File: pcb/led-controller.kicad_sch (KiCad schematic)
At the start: 39 parts, among them J1 BOOT_SEL, J2 Programmer Conn, J3 USB_C_Receptacle, SW1 PD Reset, U1 STM32F411CCUx, U2 STUSB4500QTR, Y1 16MHz

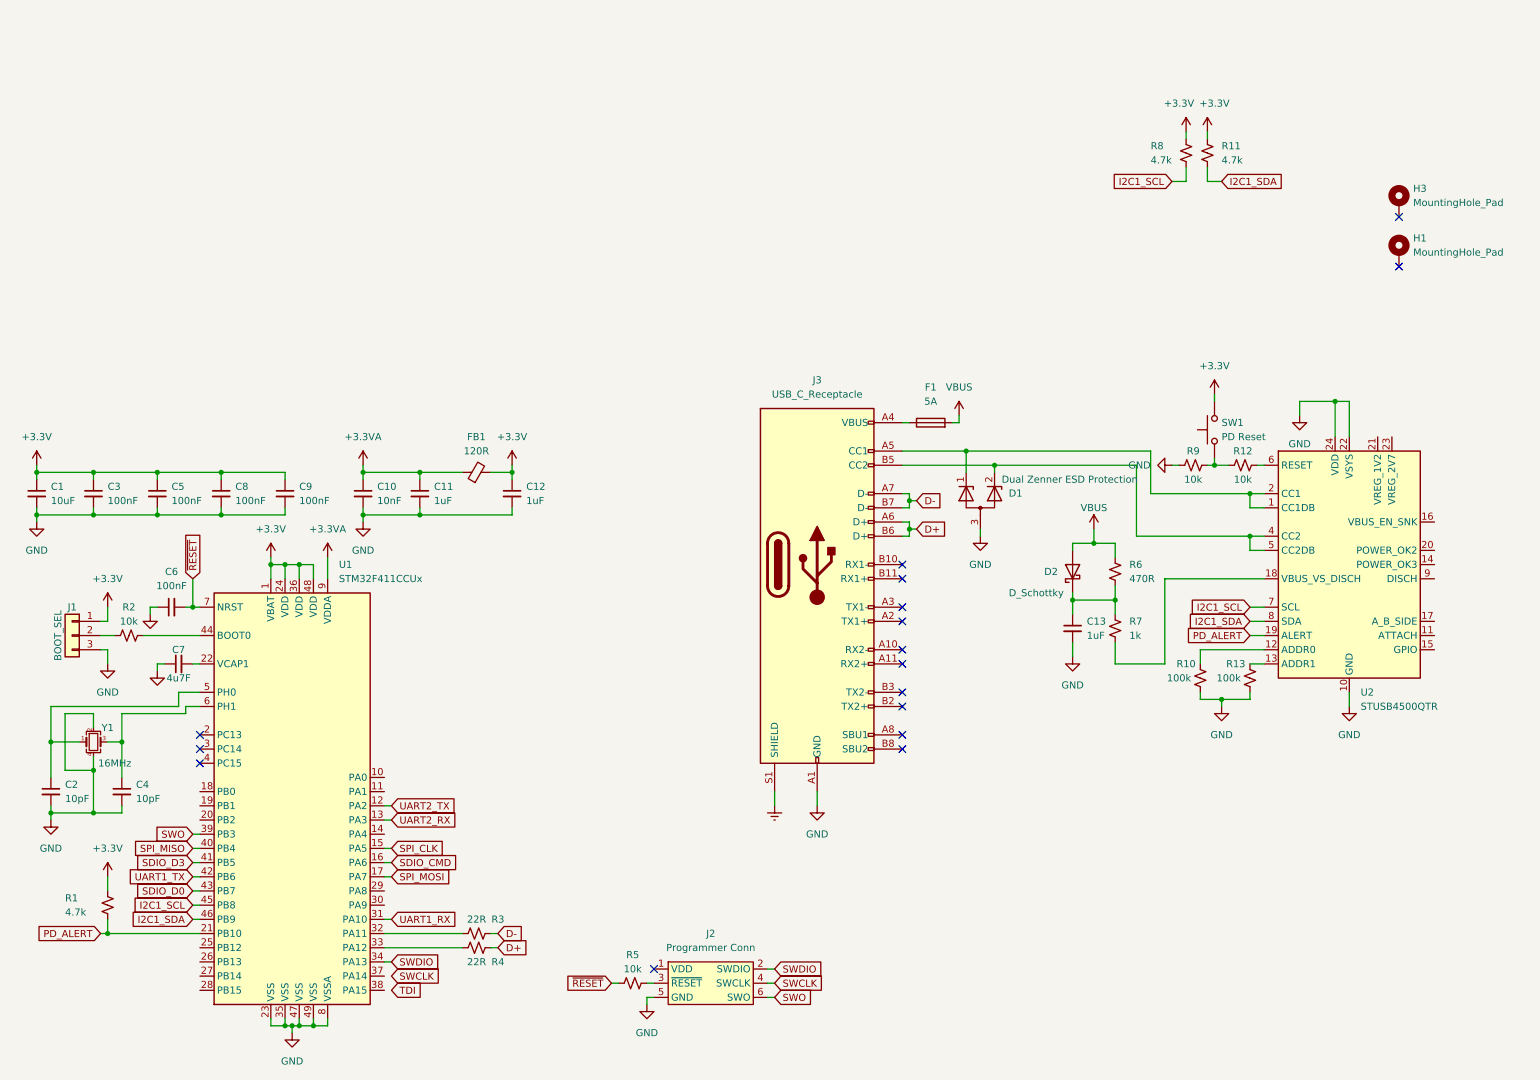
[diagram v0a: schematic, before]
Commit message: PCB updates
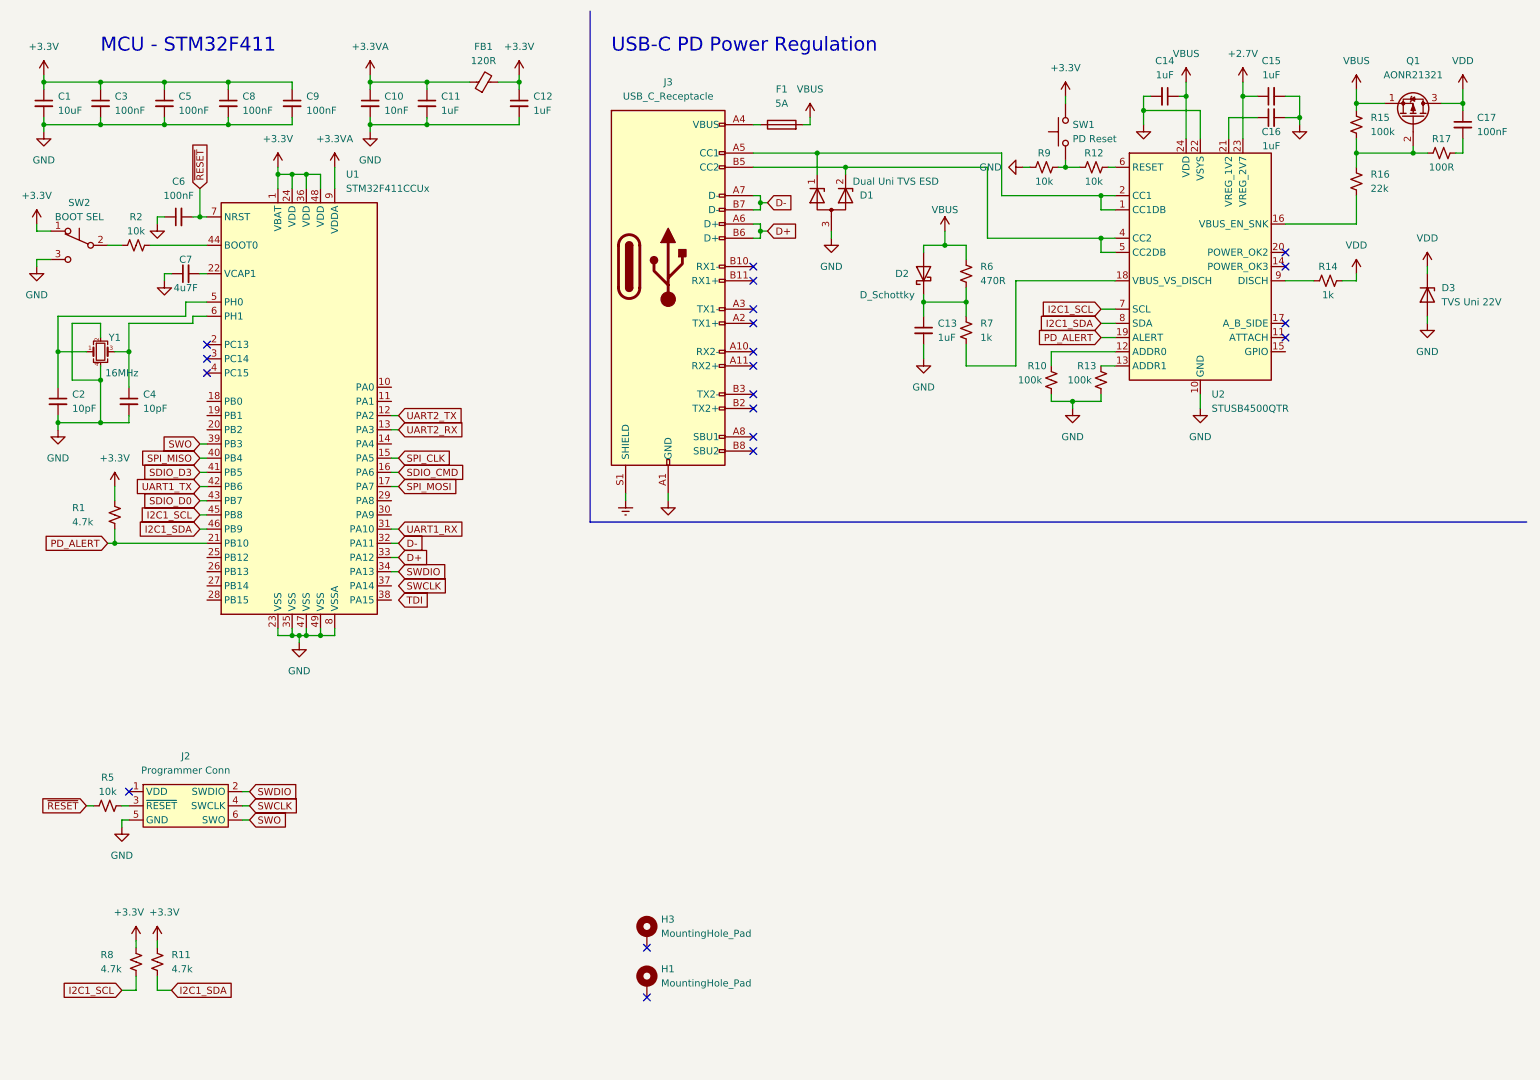
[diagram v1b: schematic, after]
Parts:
- removed J1: BOOT_SEL, Connector_PinHeader_1.27mm:PinHeader_1x03_P1.27mm_Horizontal, symbol Connector_Generic:Conn_01x03
- removed R3, R4: 22R, Resistor_SMD:R_0603_1608Metric, symbol Device:R_Small_US
- added C14, C15, C16: 1uF, Capacitor_SMD:C_0603_1608Metric, symbol Device:C_Small
- added C17: 100nF, Capacitor_SMD:C_0603_1608Metric, symbol Device:C_Small
- added D3: TVS Uni 22V, symbol Device:D_Zener
- added Q1: AONR21321, ATL:AONR21321, symbol ATL:AONR21321
- added R14: 1k, Resistor_SMD:R_0603_1608Metric, symbol Device:R_Small_US
- added R15: 100k, Resistor_SMD:R_0603_1608Metric, symbol Device:R_Small_US
- added R16: 22k, Resistor_SMD:R_0603_1608Metric, symbol Device:R_Small_US
- added R17: 100R, Resistor_SMD:R_0603_1608Metric, symbol Device:R_Small_US
- added SW2: BOOT SEL, Button_Switch_SMD:SW_DIP_SPSTx01_Slide_Copal_CVS-01xB_W5.9mm_P1mm, symbol Switch:SW_Push_SPDT
- D1: value Dual Zenner ESD Protection -> Dual Uni TVS ESD
- F1: footprint (none) -> ATL:Littlefuse-154
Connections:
- net +3.3V: now also SW2.1 (A)
- net D+: now also U1.33 (PA12)
- net D-: now also U1.32 (PA11)
- net GND: now also C14.2, C15.2, C16.2, D3.2 (A), SW2.3 (C); no longer U2.24 (VDD)
- net VBUS: now also U2.24 (VDD), C14.1, Q1.1 (S), R15.1
- net at R2.1: now also SW2.2 (B)
- net at U2.16 (VBUS_EN_SNK): now also R16.2
- net at U2.21 (VREG_1V2): now also C16.1
- net +2V7: now reaches U2.23 (VREG_2V7)
- net +2V7: now also C15.1
- net at U2.9 (DISCH): now also R14.1
- new net: Q1.2 (G), R15.2, R16.1, R17.1
- new net: C17.2, R17.2
- new net VDD: C17.1, D3.1 (K), Q1.3 (D), R14.2
- no-connect marks 16 -> 20
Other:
- note added: "MCU - STM32F411"
- note added: "USB-C PD Power Regulation"
- moved on the sheet: C1, C10, C11, C12, C13, C2, C3, C4, C5, C6, C7, C8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
